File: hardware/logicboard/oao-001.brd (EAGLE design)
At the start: 51.7 x 40.6 mm, 9 parts, among them K1 G5V1, T1 2SC1815

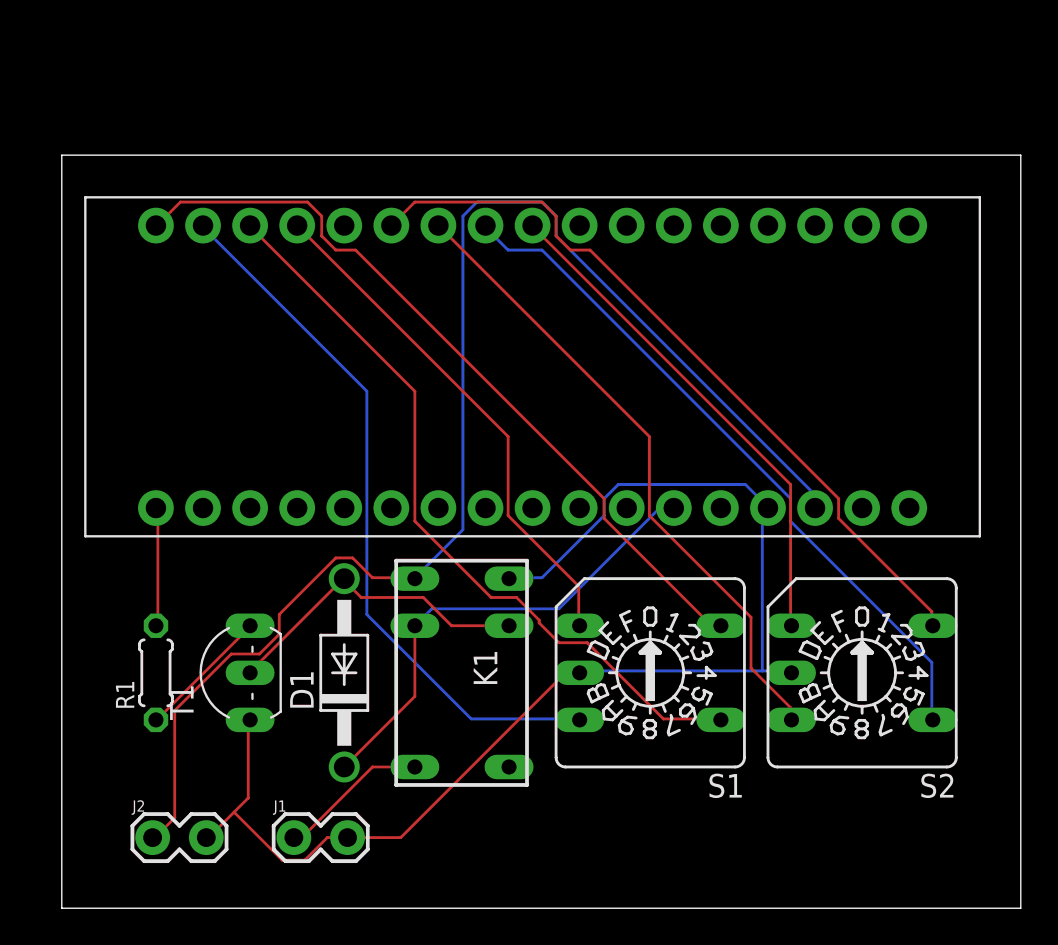
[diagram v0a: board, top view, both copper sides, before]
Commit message: Released hardware.
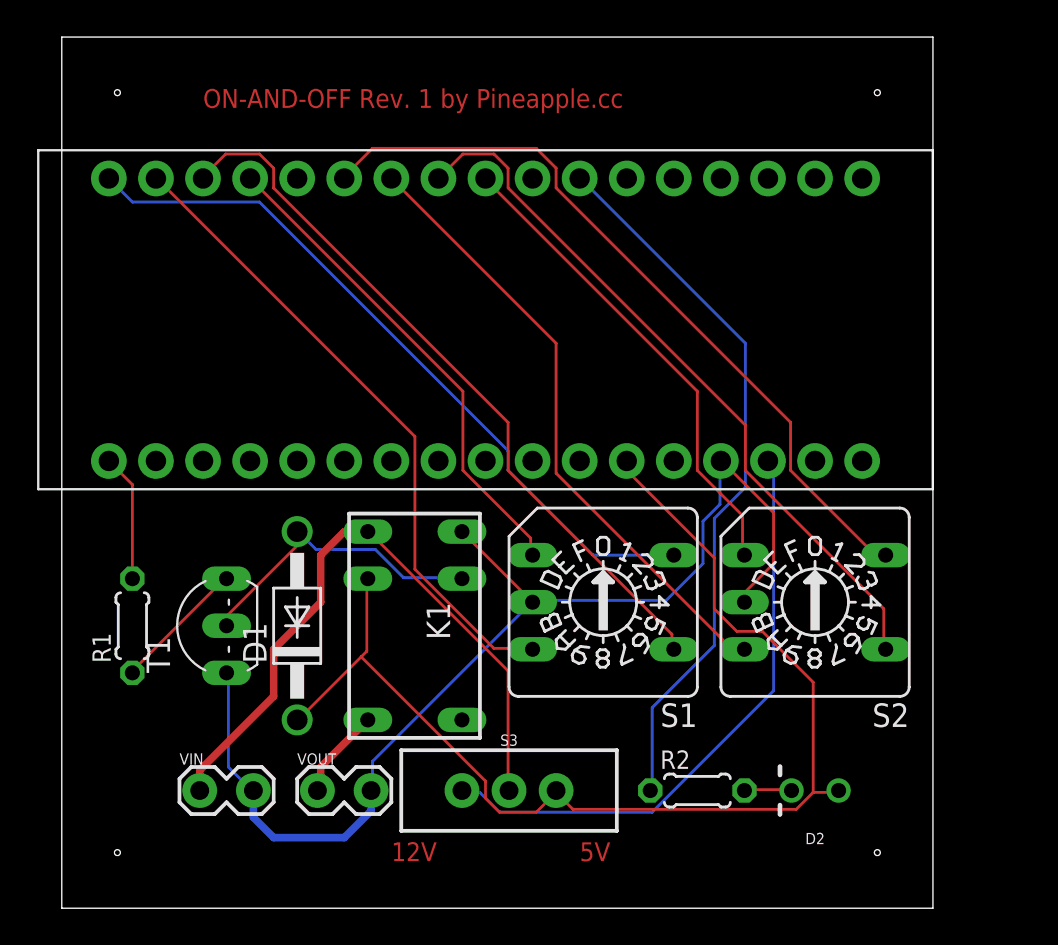
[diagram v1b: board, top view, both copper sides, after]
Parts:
- removed J1, J2: (no value), SparkFun-Connectors:1X02_LOCK
- added D2: (no value), SparkFun-LED:LED_3MM-NS
- added R2: 220, resistor:0204/5
- added S3: NC: 5V, NO: 12V, SparkFun-Switches:SWITCH_SPDT_PTH_11.6X4.0MM
- added VIN, VOUT: (no value), SparkFun-Connectors:1X02_LOCK
- R1: value (none) -> 3.3k
- moved S1 4.58 mm to (29.2, 16.5)
- moved S2 4.58 mm to (40.6, 16.5)
- moved D1 3.59 mm to (12.7, 15.2)
- moved K1 3.59 mm to (19.1, 15.2)
- moved U$1 3.59 mm to (22.9, 31.8)
- moved R1 2.84 mm to (3.81, 15.2)
- moved T1 2.84 mm to (8.89, 15.2)
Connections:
- new net N$13: R2.1, U$1.P$11
- new net N$14: D2.K, R2.2
- new net N$15: S3.3, U$1.P$20
- net GND: now also VIN.2, VOUT.2; no longer J1.2, J2.2
- net N$1: now also VOUT.1; no longer J1.1
- net VCC: now also D2.A, S3.1
- net VDD: now also S3.2, VIN.1; no longer J2.1, U$1.P$20
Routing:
- net N$13: track 0.00 -> 38.9 mm
- net VCC: track 25.8 -> 63.2 mm
- net VDD: track 72.8 -> 35.6 mm
- net N$15: track 0.00 -> 32.6 mm
- net GND: track 68.9 -> 61.6 mm
- net N$8: track 38.5 -> 35.0 mm
- net N$1: track 8.11 -> 4.94 mm
- net N$14: track 0.00 -> 2.58 mm
- net N$7: track 41.7 -> 39.5 mm
- net N$11: track 37.7 -> 39.0 mm
- net N$10: track 27.9 -> 26.7 mm
- net N$12: track 27.4 -> 26.2 mm
- net N$9: track 40.7 -> 39.7 mm
- net N$6: track 34.6 -> 33.7 mm
- net N$4: track 17.3 -> 16.6 mm
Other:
- board size 51.7 x 40.6 mm -> 47 x 47 mm
- board text added: "12V"
- board text added: "5V"
- board text added: "ON-AND-OFF Rev. 1 by Pineapple.cc"
